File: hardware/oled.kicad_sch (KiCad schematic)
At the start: 1 part, among them J17 Conn_01x30

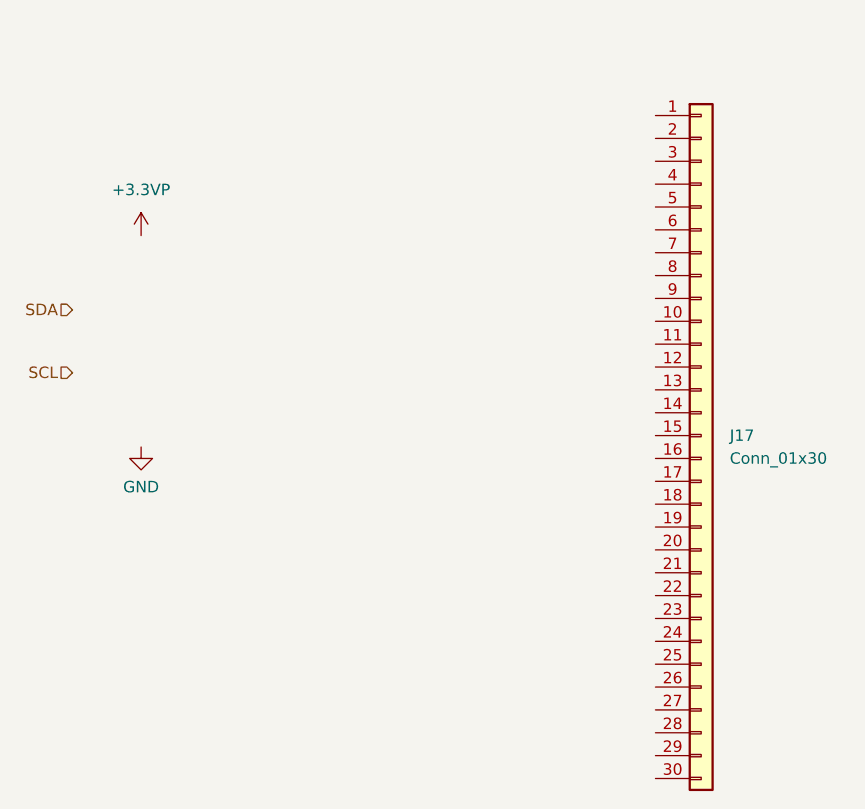
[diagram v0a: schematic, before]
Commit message: OLED regulator
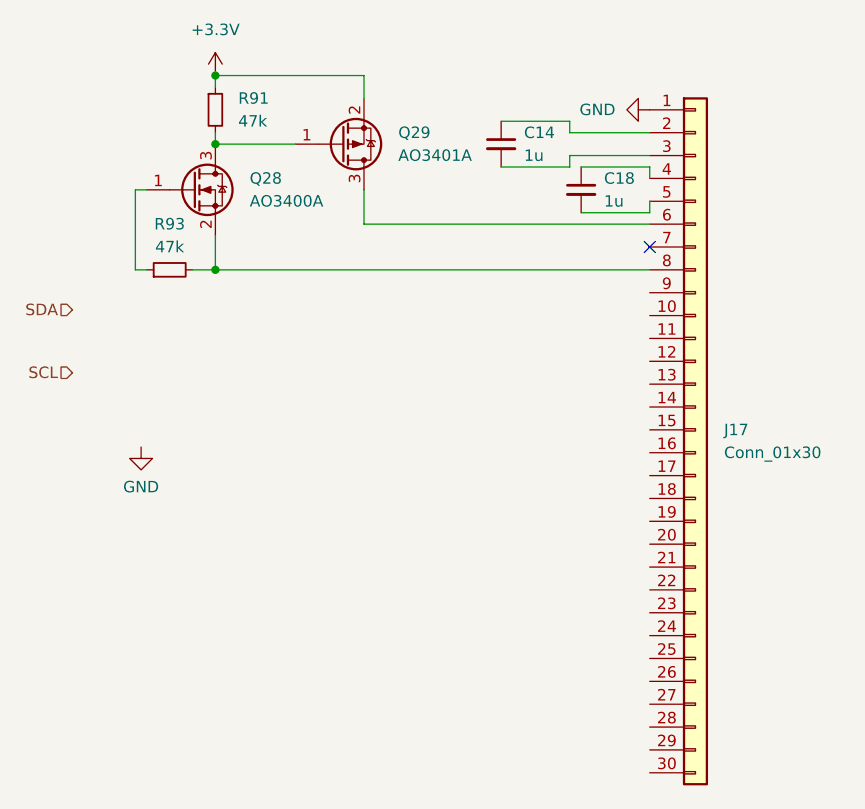
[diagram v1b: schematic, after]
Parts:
- added C14, C18: 1u, symbol Device:C_Small
- added Q28: AO3400A, Package_TO_SOT_SMD:SOT-23, symbol Transistor_FET:AO3400A
- added Q29: AO3401A, Package_TO_SOT_SMD:SOT-23, symbol Transistor_FET:AO3401A
- added R91, R93: 47k, symbol Device:R_Small
- J17: LCSC (none) -> C2890596
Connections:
- net GND: now also J17.1 (Pin_1)
- net at J17.2 (Pin_2): now also C14.1
- net at J17.3 (Pin_3): now also C14.2
- net at J17.4 (Pin_4): now also C18.1
- net at J17.5 (Pin_5): now also C18.2
- net at J17.6 (Pin_6): now also Q29.3 (D)
- net at J17.8 (Pin_8): now also Q28.2 (S), R93.2
- new net: Q28.3 (D), Q29.1 (G), R91.2
- new net: Q28.1 (G), R93.1
- new net +3.3V: Q29.2 (S), R91.1
- no-connect marks 0 -> 1
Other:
- moved on the sheet: J17
